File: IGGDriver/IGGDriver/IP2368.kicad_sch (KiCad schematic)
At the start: 23 parts, among them U16 IP2326

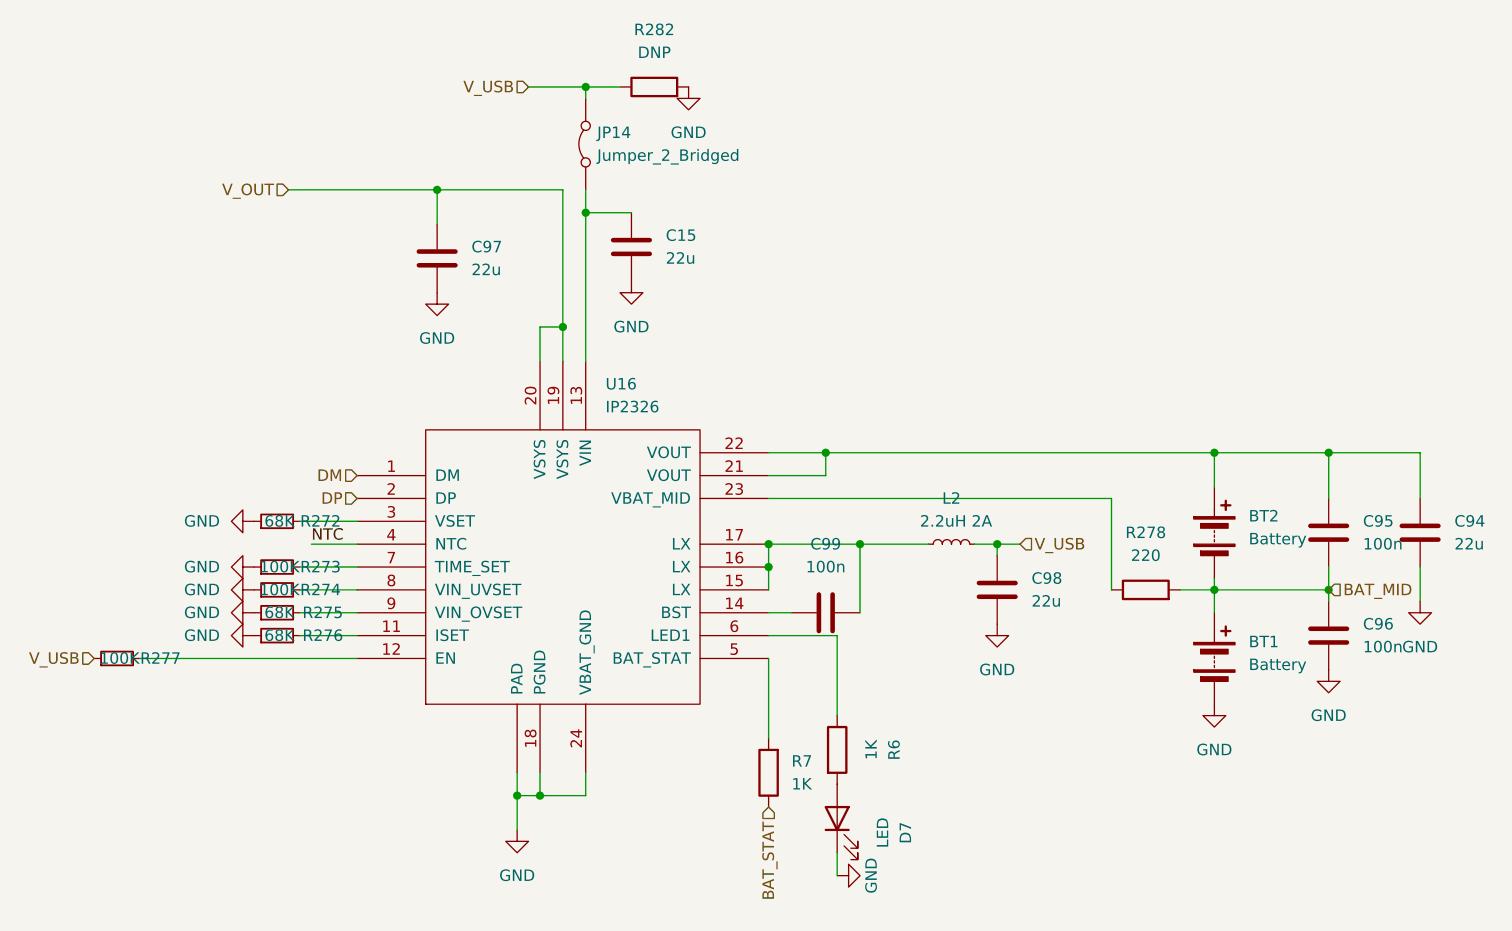
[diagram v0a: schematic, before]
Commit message: Push to other computer to edit footprint
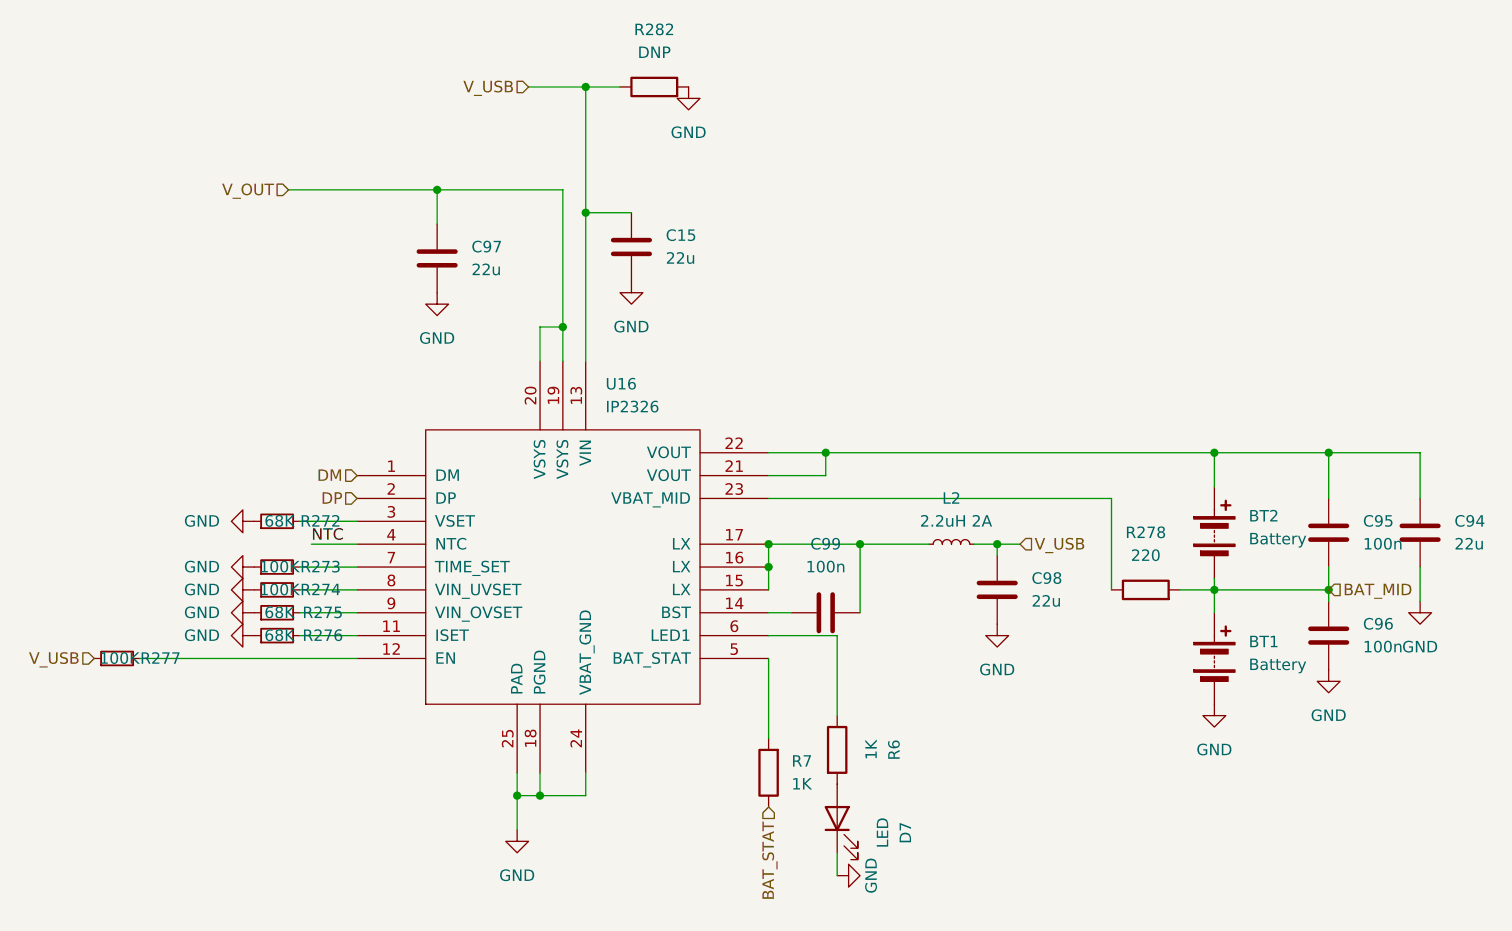
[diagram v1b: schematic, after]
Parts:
- removed JP14: Jumper_2_Bridged, symbol Jumper:Jumper_2_Bridged
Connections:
- net GND: now also U16.25 (PAD); no longer U16. (PAD)
- net V_USB: now also C15.1, U16.13 (VIN)
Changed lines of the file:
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@@
-	(wire
-		(pts
-			(xy 120.65 40.64) (xy 120.65 43.18)
-		)
-		(stroke
-			(width 0)
-			(type default)
-		)
-	)
 	(wire
 		(pts
@@
 	(wire
 		(pts
-			(xy 120.65 29.21) (xy 120.65 30.48)
+			(xy 120.65 29.21) (xy 120.65 43.18)
 		)
 		(stroke
@@
 		(pin "22"
 		)
-		(pin ""
+		(pin "25"
 		)
 		(instances
@@
 					(unit 1)
 				)
-			)
-		)
-	)
-	(symbol
-		(lib_id "Jumper:Jumper_2_Bridged")
-		(at 120.65 35.56 90)
-		(unit 1)
-		(exclude_from_sim yes)
-		(in_bom yes)
-		(on_board yes)
-		(dnp no)
-		(fields_autoplaced yes)
-		(property "Reference" "JP14"
-			(at 121.92 34.2899 90)
-			(effects
-				(font
-					(size 1.27 1.27)
-				)
-				(justify right)
-			)
-		)
-		(property "Value" "Jumper_2_Bridged"
-			(at 121.92 36.8299 90)
-			(effects
-				(font
-					(size 1.27 1.27)
-				)
-				(justify right)
-			)
-		)
-		(property "Footprint" ""
-			(at 120.65 35.56 0)
-			(effects
-				(font
-					(size 1.27 1.27)
-				)
-				(hide yes)
-			)
-		)
-		(property "Datasheet" "~"
-			(at 120.65 35.56 0)
-			(effects
-				(font
-					(size 1.27 1.27)
-				)
-				(hide yes)
-			)
-		)
-		(property "Description" "Jumper, 2-pole, closed/bridged"
-			(at 120.65 35.56 0)
-			(effects
-				(font
-					(size 1.27 1.27)
-				)
-				(hide yes)
-			)
-		)
-		(pin "1"
-		)
-		(pin "2"
-		)
-		(instances
-			(project "IGGDriver"
-				(path "/42dcdc8e-b1dc-4d4c-b3c7-96447ce841be/ed6672d7-92eb-40ce-b4cc-e5b4f765c723"
-					(reference "JP14")
-					(unit 1)
-				)
